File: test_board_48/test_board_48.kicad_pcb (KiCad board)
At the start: 2 copper layers, 100 x 100 mm, 14 parts, among them J1 Conn_01x01, J2 Conn_01x01

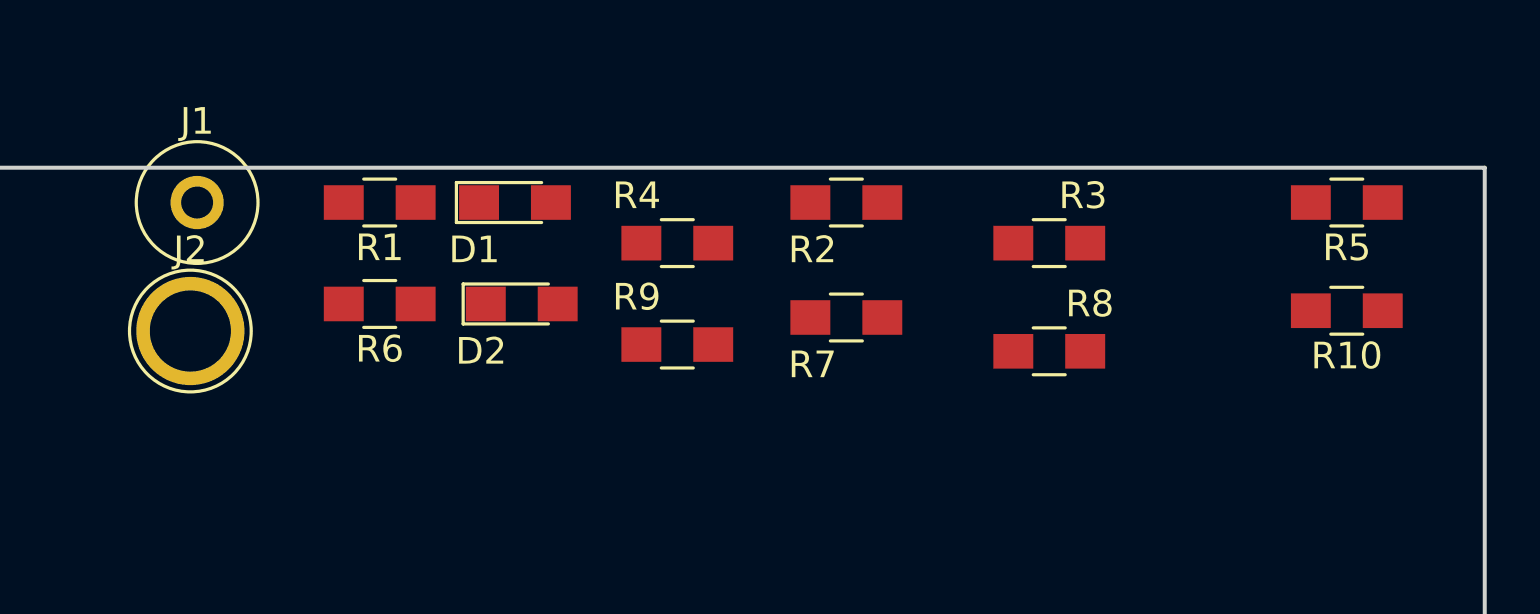
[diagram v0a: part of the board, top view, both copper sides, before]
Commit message: test board 48
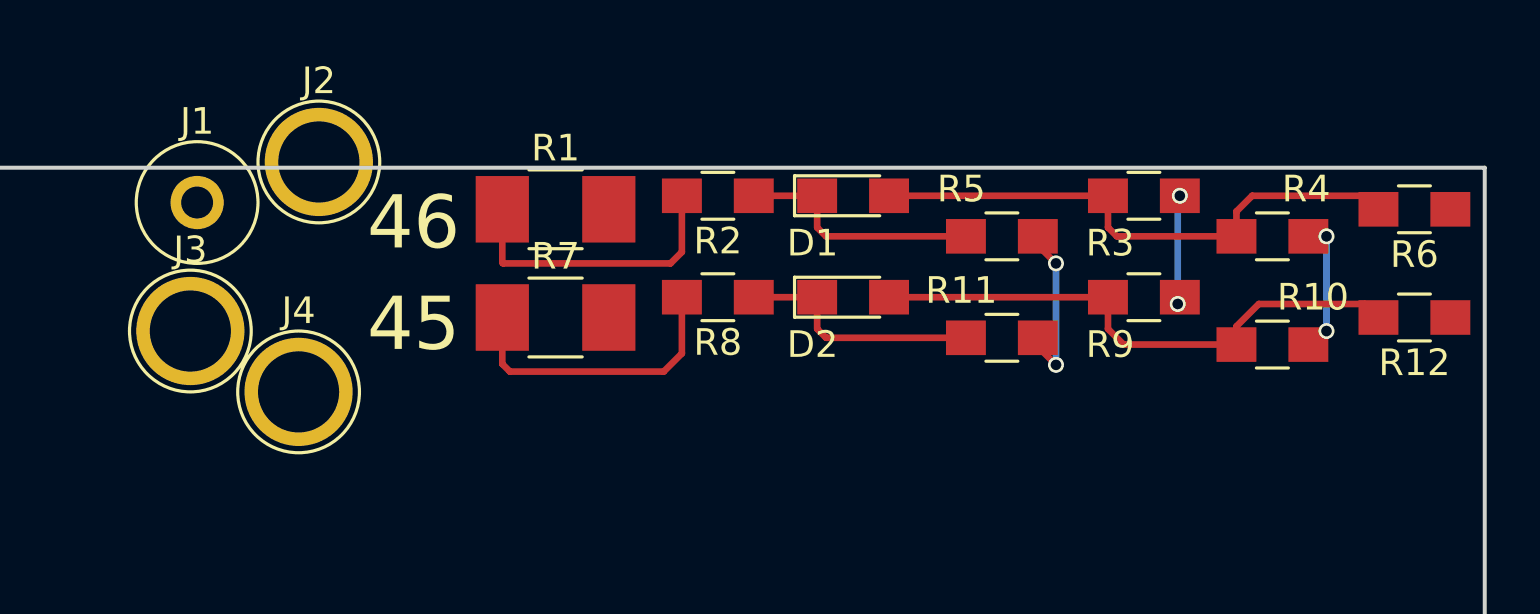
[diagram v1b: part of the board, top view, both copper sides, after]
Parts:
- added J2: Conn_01x01, Connectors:1pin, F.Cu at (156.2, 49.8)
- added J4: Conn_01x01, Connectors:1pin, F.Cu at (155.4, 58.4)
- added R1: R, Resistors_SMD:R_1210_HandSoldering, F.Cu at (165.1, 51.6)
- added R7: R, Resistors_SMD:R_1210_HandSoldering, F.Cu at (165.1, 55.6)
- moved D1 12.7 mm to (176.3, 51.1)
- moved R2 12.7 mm to (171.2, 51.1)
- moved R8 12.7 mm to (171.2, 54.9)
- moved D2 12.4 mm to (176.3, 54.9)
- moved R11 12.2 mm to (181.9, 56.4)
- moved R5 12.2 mm to (181.9, 52.6)
- moved R9 11.2 mm to (187.2, 54.9)
- moved R3 11.2 mm to (187.2, 51.1)
- moved R10 8.39 mm to (192.0, 56.6)
- moved R4 8.39 mm to (192.0, 52.6)
- moved R12 2.55 mm to (197.4, 55.6)
- moved R6 2.55 mm to (197.4, 51.6)
- renumbered J2 to J3, R8 to R10, R9 to R11, R10 to R12, R1 to R2, R2 to R3, R3 to R4, R4 to R5, R5 to R6, R6 to R8, R7 to R9
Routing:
- net Net-(D1-Pad2): track 0.00 -> 21.8 mm
- net Net-(D2-Pad2): track 0.00 -> 21.8 mm
- net Net-(J1-Pad1): track 0.00 -> 11.0 mm
- net Net-(J3-Pad1): track 0.00 -> 11.0 mm
- net Net-(D2-Pad1): track 0.00 -> 9.30 mm
- net Net-(D1-Pad1): track 0.00 -> 9.30 mm
- net GND: track 0.00 -> 6.41 mm, vias 0 -> 2
- net /12v: track 0.00 -> 4.96 mm, vias 0 -> 2
- net /5v: track 0.00 -> 4.38 mm, vias 0 -> 2
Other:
- board text added: "45"
- board text added: "46"
